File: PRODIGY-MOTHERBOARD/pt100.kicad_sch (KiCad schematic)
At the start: 5 parts, among them U10 LMP2011, U11 LMP2011, U17 LMP2011, U27 LMP2011, U9 LM4125AIM5-2.5

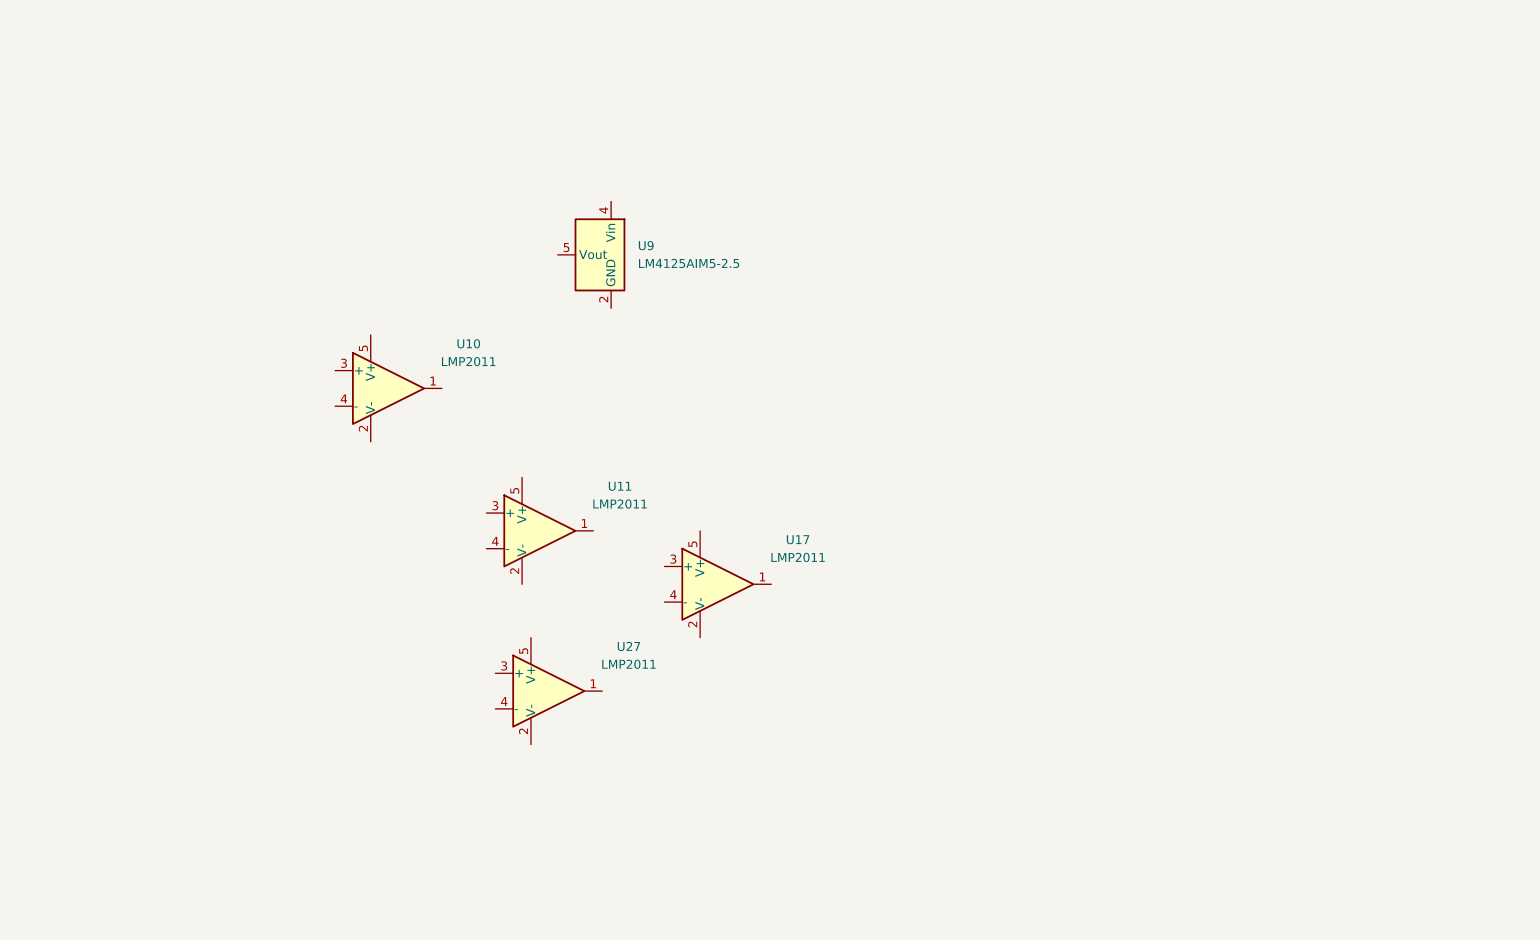
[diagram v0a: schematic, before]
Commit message: Finished v0.1 schematic.
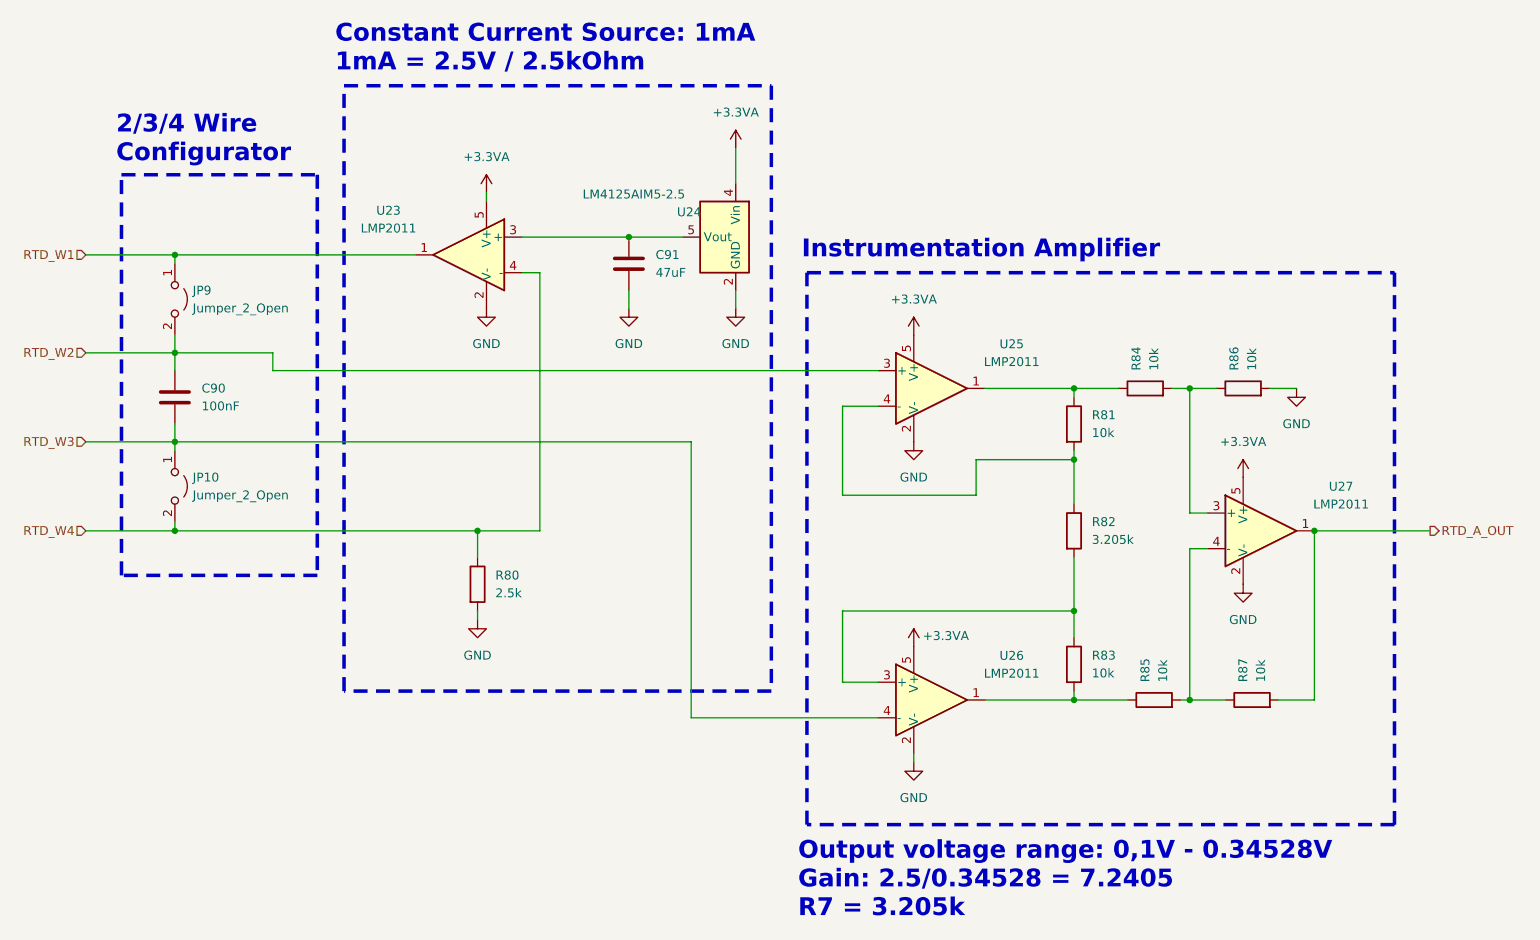
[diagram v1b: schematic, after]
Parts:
- added C90: 100nF, symbol Device:C
- added C91: 47uF, symbol Device:C
- added JP10, JP9: Jumper_2_Open, symbol Jumper:Jumper_2_Open
- added R80: 2.5k, symbol Device:R
- added R81, R83, R84, R85, R86, R87: 10k, symbol Device:R
- added R82: 3.205k, symbol Device:R
- renumbered U10 to U23, U9 to U24, U11 to U25, U17 to U26
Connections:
- net at U26.1: now also R83.2, R85.1
- net GND: now reaches U26.2 (V-)
- net GND: now also U23.2 (V-), U24.2 (GND), U25.2 (V-), U27.2 (V-), C91.2, R80.2, R86.2
- net at U26.3 (+): now also R82.2, R83.1
- net RTD_W3: now reaches U26.4 (-)
- net RTD_W3: now also C90.2, JP10.1 (A)
- net +3.3VA: now reaches U26.5 (V+)
- net +3.3VA: now also U23.5 (V+), U24.4 (Vin), U25.5 (V+), U27.5 (V+)
- net RTD_A_OUT: now reaches U27.1
- net RTD_A_OUT: now also R87.2
- net at U27.3 (+): now also R84.2, R86.1
- net at U27.4 (-): now also R85.2, R87.1
- net at U24.5 (Vout): now also U23.3 (+), C91.1
- net RTD_W1: now reaches U23.1
- net RTD_W1: now also JP9.1 (A)
- net RTD_W4: now reaches U23.4 (-)
- net RTD_W4: now also JP10.2 (B), R80.1
- net at U25.1: now also R81.1, R84.1
- net RTD_W2: now reaches U25.3 (+)
- net RTD_W2: now also C90.1, JP9.2 (B)
- net at U25.4 (-): now also R81.2, R82.1
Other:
- note added: "2/3/4 Wire Configurator"
- note added: "Constant Current Source: 1mA 1mA = 2.5V / 2.5kOhm"
- note added: "Instrumentation Amplifier"
- note added: "Output voltage range: 0,1V - 0.34528V Gain: 2.5/0.34528 = 7.2405 R7 = 3.205k"
- moved on the sheet: U23, U24, U25, U26, U27
